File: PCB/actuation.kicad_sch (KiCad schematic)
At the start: 3 parts, among them U4 TCA0372_DWG

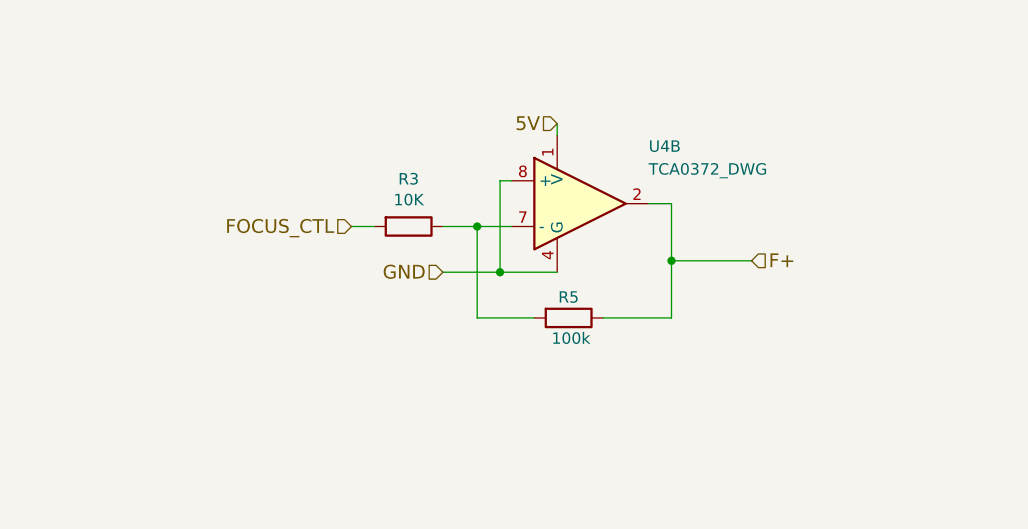
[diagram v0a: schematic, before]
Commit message: Modify PCB
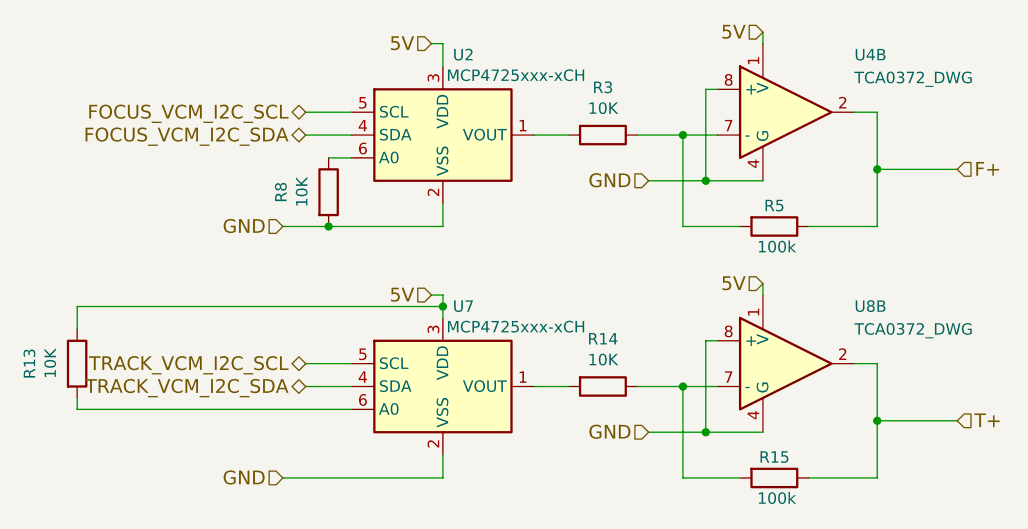
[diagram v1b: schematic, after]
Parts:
- added R13, R14, R8: 10K, GaudiLabsFootPrints:0805G, symbol DVDLaserScanner-rescue:R
- added R15: 100k, GaudiLabsFootPrints:0805G, symbol DVDLaserScanner-rescue:R
- added U2, U7: MCP4725xxx-xCH, Package_TO_SOT_SMD:SOT-23-6, symbol Analog_DAC:MCP4725xxx-xCH
- added U8: TCA0372_DWG, GaudiLabsFootPrints:SO-16-W, symbol DVDLaserScanner-rescue:TCA0372_DWG
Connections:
- net 5V: now also R13.1, U2.3 (VDD), U7.3 (VDD), U8.1 (V)
- net GND: now also R8.2, U2.2 (VSS), U7.2 (VSS), U8.12 (GND), U8.13 (GND), U8.4 (G), U8.5 (GND), U8.8 (+)
- net FOCUS_CTL: no longer names the net of R3.2
- net FOCUS_CTL: now also U2.1 (VOUT)
- new net: R8.1, U2.6 (A0)
- new net: R14.2, U7.1 (VOUT)
- new net: R13.2, U7.6 (A0)
- new net: R14.1, R15.2, U8.7 (-)
- new net FOCUS_VCM_I2C_SCL: U2.5 (SCL)
- new net FOCUS_VCM_I2C_SDA: U2.4 (SDA)
- new net T+: R15.1, U8.2
- new net TRACK_VCM_I2C_SCL: U7.5 (SCL)
- new net TRACK_VCM_I2C_SDA: U7.4 (SDA)
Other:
- moved on the sheet: R3, R5, U4B
